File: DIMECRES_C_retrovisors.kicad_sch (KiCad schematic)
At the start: 96 parts, among them J10 Vbat, J2 DE9_Pins, J3 Conn_01x05_Pin, J4 Motor3, J5 DE9_Pins, J6 Intermitente, J7 Calentador, J8 Motor2, J9 Motor1, Q1 DTC144E, Q2 DTC144E, Q3 DTC144E, SW1 SW_DPDT_G6S, SW10 SW_Push, SW2 SW_Push, SW3 SW_Push, SW4 SW_Push, SW5 SW_Push, SW6 SW_Push, SW7 SW_Push, SW8 FN01B, SW9 FN01B, U1 CH201, U10 LM1117DT-5.0, U2 ADM7160, U3 LM2596S-ADJ, U4 L298N, U5 MCP2551-I-SN, U6 ADA4511-2, U7 PIC18F4480-IP, U8 LSF0002, Y1 Crystal

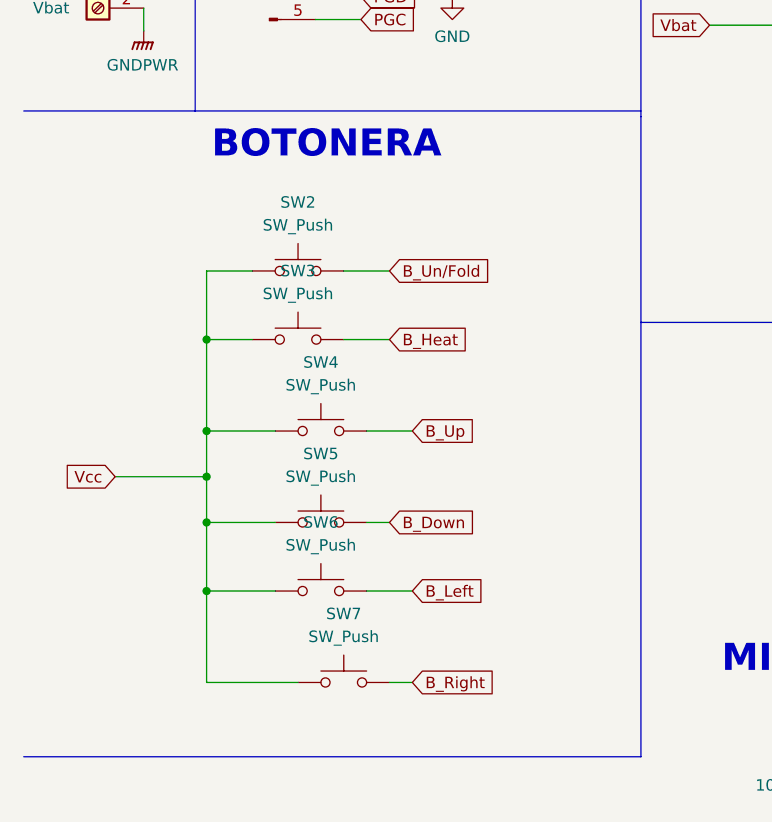
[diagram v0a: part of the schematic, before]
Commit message: De to
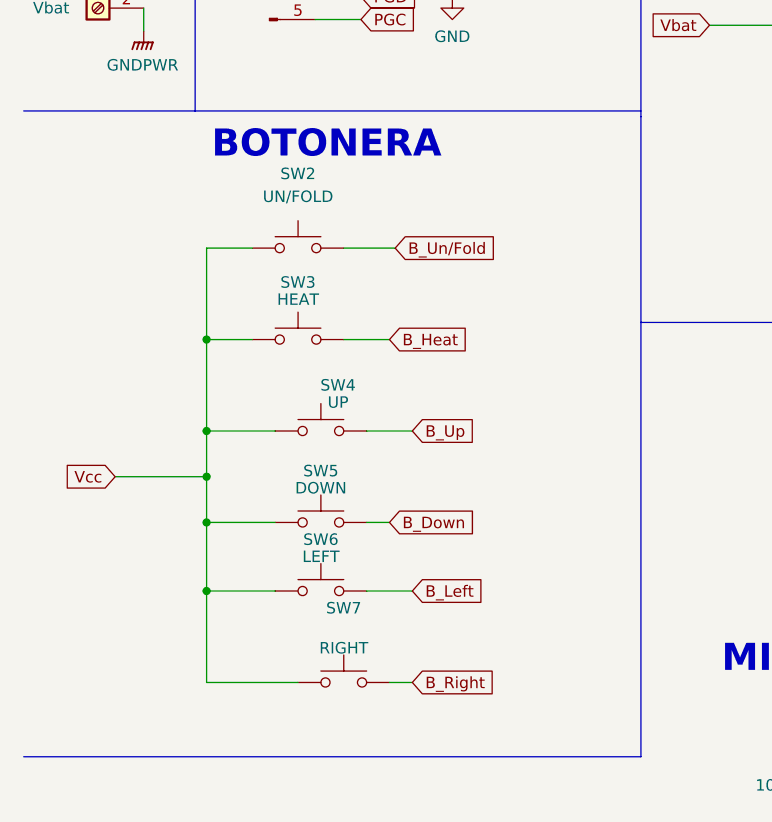
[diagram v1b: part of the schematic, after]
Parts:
- C23: footprint Capacitor_SMD:C_1206_3216Metric_Pad1.33x1.80mm_HandSolder -> Capacitor_SMD:C_0805_2012Metric_Pad1.18x1.45mm_HandSolder
- R10, R11, R25, R26: footprint Resistor_SMD:R_1206_3216Metric_Pad1.30x1.75mm_HandSolder -> Resistor_SMD:R_0805_2012Metric_Pad1.20x1.40mm_HandSolder
- SW2: value SW_Push -> UN/FOLD
- SW3: value SW_Push -> HEAT
- SW4: value SW_Push -> UP
- SW5: value SW_Push -> DOWN
- SW6: value SW_Push -> LEFT
- SW7: value SW_Push -> RIGHT
- U10: footprint Package_TO_SOT_SMD:TO-252-3_TabPin2 -> Package_TO_SOT_SMD:TO-263-3_TabPin2
- U8: footprint (none) -> PracticasKiCad:LSF0002
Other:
- moved on the sheet: SW2
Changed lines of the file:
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@@
 	(wire
 		(pts
-			(xy 33.02 67.945) (xy 38.1 67.945)
+			(xy 33.02 65.405) (xy 38.1 65.405)
 		)
 		(stroke
@@
 	(wire
 		(pts
-			(xy 53.34 67.945) (xy 48.26 67.945)
+			(xy 48.26 65.405) (xy 53.975 65.405)
 		)
 		(stroke
@@
 	(wire
 		(pts
-			(xy 33.02 67.945) (xy 33.02 75.565)
+			(xy 33.02 65.405) (xy 33.02 75.565)
 		)
 		(stroke
@@
 	(global_label "B_Un{slash}Fold"
 		(shape input)
-		(at 53.34 67.945 0)
+		(at 53.975 65.405 0)
 		(fields_autoplaced yes)
 		(effects
@@
 		)
 		(property "Intersheetrefs" "${INTERSHEET_REFS}"
-			(at 66.4246 67.945 0)
+			(at 67.0596 65.405 0)
 			(effects
 				(font
@@
 			)
 		)
-		(property "Footprint" "Resistor_SMD:R_1206_3216Metric_Pad1.30x1.75mm_HandSolder"
+		(property "Footprint" "Resistor_SMD:R_0805_2012Metric_Pad1.20x1.40mm_HandSolder"
 			(at 222.758 130.81 90)
 			(effects
@@
 			)
 		)
-		(property "Footprint" "Capacitor_SMD:C_1206_3216Metric_Pad1.33x1.80mm_HandSolder"
+		(property "Footprint" "Capacitor_SMD:C_0805_2012Metric_Pad1.18x1.45mm_HandSolder"
 			(at 213.0552 133.985 0)
 			(effects
@@
 			)
 		)
-		(property "Footprint" "Resistor_SMD:R_1206_3216Metric_Pad1.30x1.75mm_HandSolder"
+		(property "Footprint" "Resistor_SMD:R_0805_2012Metric_Pad1.20x1.40mm_HandSolder"
 			(at 232.918 130.81 90)
 			(effects
@@
 	(symbol
 		(lib_id "Switch:SW_Push")
-		(at 43.18 67.945 0)
+		(at 43.18 65.405 0)
 		(unit 1)
 		(exclude_from_sim no)
@@
 		(fields_autoplaced yes)
 		(property "Reference" "SW2"
-			(at 43.18 60.325 0)
+			(at 43.18 57.15 0)
 			(effects
 				(font
@@
 			)
 		)
-		(property "Value" "SW_Push"
-			(at 43.18 62.865 0)
+		(property "Value" "UN/FOLD"
+			(at 43.18 59.69 0)
 			(effects
 				(font
@@
 		)
 		(property "Footprint" "Button_Switch_SMD:SW_SPST_PTS647_Sx38"
-			(at 43.18 62.865 0)
+			(at 43.18 60.325 0)
 			(effects
 				(font
@@
 		)
 		(property "Datasheet" "~"
-			(at 43.18 62.865 0)
+			(at 43.18 60.325 0)
 			(effects
 				(font
@@
 		)
 		(property "Description" "Push button switch, generic, two pins"
-			(at 43.18 67.945 0)
+			(at 43.18 65.405 0)
 			(effects
 				(font
@@
 		(on_board yes)
 		(dnp no)
-		(fields_autoplaced yes)
 		(property "Reference" "SW4"
-			(at 45.72 78.105 0)
+			(at 47.625 80.645 0)
 			(effects
 				(font
@@
 			)
 		)
-		(property "Value" "SW_Push"
-			(at 45.72 80.645 0)
+		(property "Value" "UP"
+			(at 47.625 82.55 0)
 			(effects
 				(font
@@
 		(on_board yes)
 		(dnp no)
-		(fields_autoplaced yes)
 		(property "Reference" "SW6"
-			(at 45.72 95.885 0)
+			(at 45.72 97.79 0)
 			(effects
 				(font
@@
 			)
 		)
-		(property "Value" "SW_Push"
-			(at 45.72 98.425 0)
+		(property "Value" "LEFT"
+			(at 45.72 99.695 0)
 			(effects
 				(font
@@
 			)
 		)
-		(property "Footprint" "Resistor_SMD:R_1206_3216Metric_Pad1.30x1.75mm_HandSolder"
+		(property "Footprint" "Resistor_SMD:R_0805_2012Metric_Pad1.20x1.40mm_HandSolder"
 			(at 180.213 132.08 90)
 			(effects
@@
 			)
 		)
-		(property "Footprint" "Package_TO_SOT_SMD:TO-252-3_TabPin2"
+		(property "Footprint" "Package_TO_SOT_SMD:TO-263-3_TabPin2"
 			(at 187.96 45.72 0)
 			(effects
@@
 		(on_board yes)
 		(dnp no)
-		(fields_autoplaced yes)
 		(property "Reference" "SW7"
-			(at 48.26 106.045 0)
+			(at 48.26 105.41 0)
 			(effects
 				(font
@@
 			)
 		)
-		(property "Value" "SW_Push"
-			(at 48.26 108.585 0)
+		(property "Value" "RIGHT"
+			(at 48.26 109.855 0)
 			(effects
 				(font
@@
 			)
 		)
-		(property "Footprint" "Resistor_SMD:R_1206_3216Metric_Pad1.30x1.75mm_HandSolder"
+		(property "Footprint" "Resistor_SMD:R_0805_2012Metric_Pad1.20x1.40mm_HandSolder"
 			(at 170.053 132.08 90)
 			(effects
@@
 		(on_board yes)
 		(dnp no)
-		(fields_autoplaced yes)
 		(property "Reference" "SW3"
-			(at 43.18 67.945 0)
+			(at 43.18 69.215 0)
 			(effects
 				(font
@@
 			)
 		)
-		(property "Value" "SW_Push"
-			(at 43.18 70.485 0)
+		(property "Value" "HEAT"
+			(at 43.18 71.12 0)
 			(effects
 				(font
@@
 		(on_board yes)
 		(dnp no)
-		(fields_autoplaced yes)
 		(property "Reference" "SW5"
-			(at 45.72 88.265 0)
+			(at 45.72 90.17 0)
 			(effects
 				(font
@@
 			)
 		)
-		(property "Value" "SW_Push"
-			(at 45.72 90.805 0)
+		(property "Value" "DOWN"
+			(at 45.72 92.075 0)
 			(effects
 				(font
@@
 			)
 		)
-		(property "Footprint" ""
+		(property "Footprint" "PracticasKiCad:LSF0002"
 			(at 190.5 139.7 0)
 			(effects
